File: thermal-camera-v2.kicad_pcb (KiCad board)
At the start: 4 copper layers, 46.3 x 84.7 mm, 121 parts, among them J1 Raspberry_Pi_2_3, J2 Screw_Terminal_M2_L10, J3 Screw_Terminal_M2_L10, J4 Conn_02x04_Odd_Even, J5 Conn_01x03, J6 Screw_Terminal_01x01, U1 ATtiny1616-M, U10 ME6216A28XG, U12 3N25000G33YC, U13 TD6810, U14 TD6810, U15 MMC5633NJL, U16 Ai-Thinker-Ra-01, U2 SHT30-DIS, U3 SIM7600G-H-M.2, U4 ME6211, U5 Flir_LEPTON, U6 SPH0645LM4H, U7 PCF8563T, U8 Antenna_1002427, U9 MAX98357, Y1 Crystal

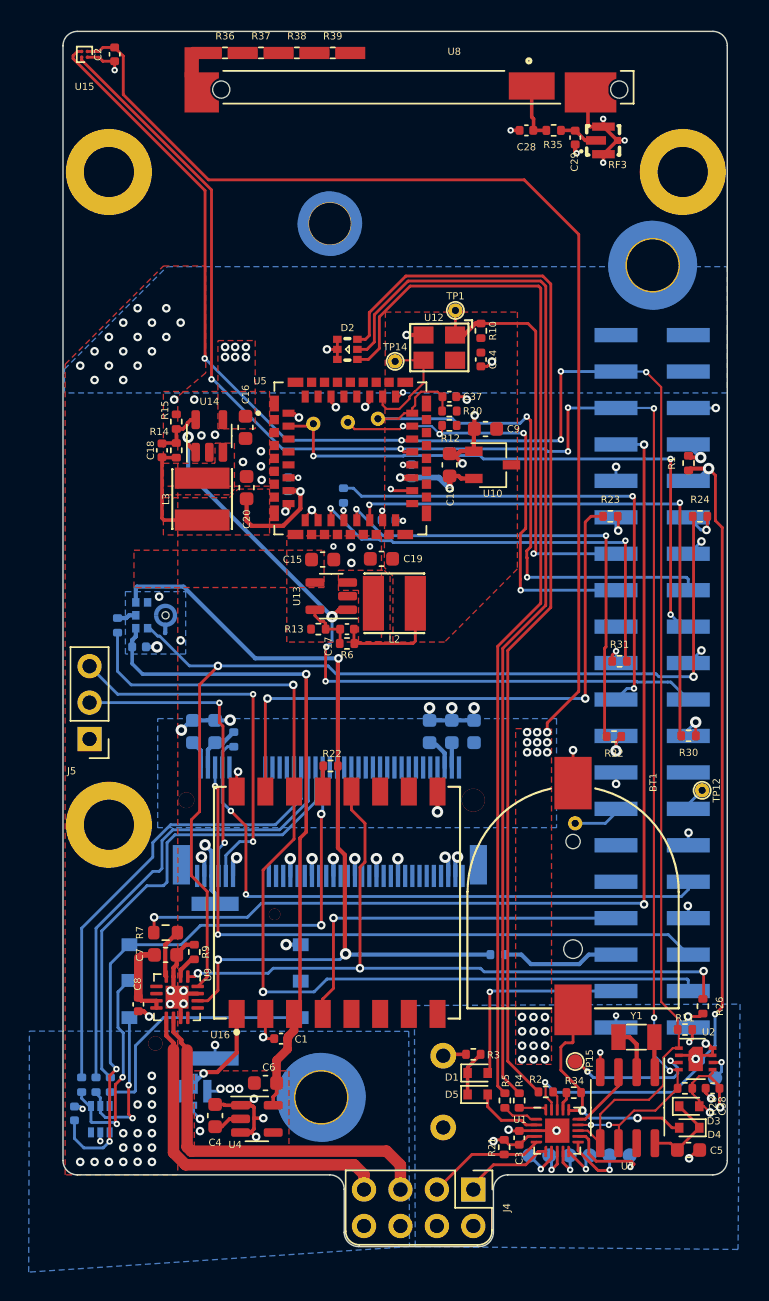
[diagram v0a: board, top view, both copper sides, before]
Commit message: WIP
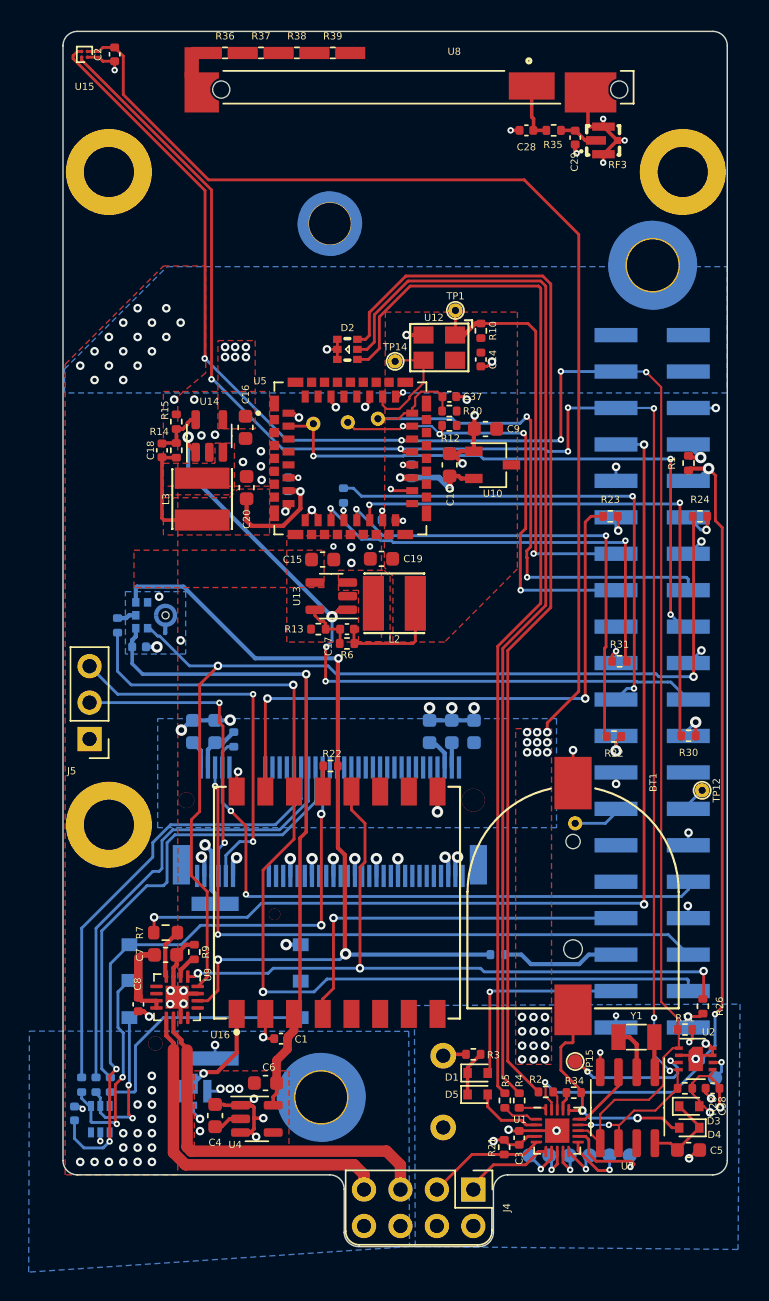
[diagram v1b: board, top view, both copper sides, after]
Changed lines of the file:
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@@
     (pad "32" smd rect (at -3.15 -4.31) (size 0.5 0.84) (layers "F.Cu" "F.Paste" "F.Mask")
       (net 133 "unconnected-(U5-Pad32)") (pinfunction "MIPI_DATA_P") (pintype "output+no_connect"))
+    (model "/home/cam/Downloads/105028-1001.stp"
+      (offset (xyz 0 0 2.1))
+      (scale (xyz 1 1 1))
+      (rotate (xyz -90 0 0))
+    )
   )
   (footprint "cacophony-library:TP" (layer "F.Cu")
@@
       (options (clearance outline) (anchor circle))
       (primitives
-    (gr_arc (start 1.238687 2.158493) (mid 0.331674 1.24433) (end 0 0) (width 1.2))
+    (gr_arc (start 1.238687 2.158493) (mid 0.332763 1.246221) (end 0.000008 0.004362) (width 1.2))
       ))
     (pad "1" smd custom (at 0 -2.5 180) (size 0.1 0.1) (layers "B.Cu" "B.Paste" "B.Mask")
@@
       (options (clearance outline) (anchor circle))
       (primitives
-    (gr_arc (start 1.234921 2.156287) (mid 0.330589 1.242437) (end 0 0) (width 1.2))
+    (gr_arc (start 1.234921 2.156287) (mid 0.332763 1.246219) (end 0.00002 0.008724) (width 1.2))
       ))
     (pad "1" smd custom (at 0 2.5) (size 0.1 0.1) (layers "B.Cu" "B.Paste" "B.Mask")
@@
       (options (clearance outline) (anchor circle))
       (primitives
-    (gr_arc (start 1.238686 2.158492) (mid 0.331673 1.24433) (end 0 0) (width 1.2))
+    (gr_arc (start 1.238686 2.158492) (mid 0.332761 1.246224) (end 0.000004 0.004369) (width 1.2))
       ))
     (pad "1" smd circle (at 0 0 270) (size 6.2 6.2) (layers "B.Cu" "B.Mask")
@@
       (options (clearance outline) (anchor circle))
       (primitives
-    (gr_arc (start 1.234922 2.156288) (mid 0.330589 1.242438) (end 0 0) (width 1.2))
+    (gr_arc (start 1.234922 2.156288) (mid 0.33059 1.242441) (end 0 0.000007) (width 1.2))
       ))
     (pad "1" thru_hole circle (at 0 0 270) (size 3.8 3.8) (drill 3.6) (layers *.Cu *.Mask)
@@
       (rotate (xyz 0 0 0))
     )
-    (model "${CAC_KICAD_LIBRARY}/cacophony-library.3dshapes/RaspberryPi3B.step"
+    (model "${CAC_KICAD_LIBRARY}/cacophony-library.3dshapes/RaspberryPi3B.step" hide
       (offset (xyz 0 0 26))
       (scale (xyz 1 1 1))
@@
       (options (clearance outline) (anchor circle))
       (primitives
-    (gr_arc (start 1.238686 2.158492) (mid 0.331673 1.24433) (end 0 0) (width 1.2))
+    (gr_arc (start 1.238686 2.158492) (mid 0.332761 1.246224) (end 0.000004 0.004369) (width 1.2))
       ))
     (pad "1" smd custom (at -2.5 0 270) (size 0.1 0.1) (layers "B.Cu" "B.Paste" "B.Mask")
@@
       (options (clearance outline) (anchor circle))
       (primitives
-    (gr_arc (start 1.238687 2.158493) (mid 0.331674 1.24433) (end 0 0) (width 1.2))
+    (gr_arc (start 1.238687 2.158493) (mid 0.332763 1.246221) (end 0.000008 0.004362) (width 1.2))
       ))
     (pad "1" smd custom (at 0 -2.5 180) (size 0.1 0.1) (layers "B.Cu" "B.Paste" "B.Mask")
@@
       (options (clearance outline) (anchor circle))
       (primitives
-    (gr_arc (start 1.234921 2.156287) (mid 0.330589 1.242437) (end 0 0) (width 1.2))
+    (gr_arc (start 1.234921 2.156287) (mid 0.332763 1.246219) (end 0.00002 0.008724) (width 1.2))
       ))
     (pad "1" thru_hole circle (at 0 0 270) (size 3.8 3.8) (drill 3.6) (layers *.Cu *.Mask)
@@
       (options (clearance outline) (anchor circle))
       (primitives
-    (gr_arc (start 1.234922 2.156288) (mid 0.330589 1.242438) (end 0 0) (width 1.2))
+    (gr_arc (start 1.234922 2.156288) (mid 0.33059 1.242441) (end 0 0.000007) (width 1.2))
       ))
     (model "${CAC_KICAD_LIBRARY}/cacophony-library.3dshapes/SMD_BD4.4-L4.4-D2.8.wrl"
@@
   (gr_arc (start 130.8 135.4) (mid 130.507107 136.107107) (end 129.8 136.4) (layer "Edge.Cuts") (width 0.1))
   (gr_arc (start 147.1 130.4) (mid 146.807107 131.107107) (end 146.1 131.4) (layer "Edge.Cuts") (width 0.1))
+  (dimension (type aligned) (layer "User.2")
+    (pts (xy 144 61.5) (xy 104 61.5))
+    (height 22.95)
+    (gr_text "40.0000 mm" (at 124 37.4) (layer "User.2")
+      (effects (font (size 1 1) (thickness 0.15)))
+    )
+    (format (units 3) (units_format 1) (precision 4))
+    (style (thickness 0.15) (arrow_length 1.27) (text_position_mode 0) (extension_height 0.58642) (extension_offset 0.5) keep_text_aligned)
+  )
+  (dimension (type aligned) (layer "User.2")
+    (pts (xy 104 61.5) (xy 104 107))
+    (height 21.299999)
+    (gr_text "45.5000 mm" (at 81.550001 84.25 90) (layer "User.2")
+      (effects (font (size 1 1) (thickness 0.15)))
+    )
+    (format (units 3) (units_format 1) (precision 4))
+    (style (thickness 0.15) (arrow_length 1.27) (text_position_mode 0) (extension_height 0.58642) (extension_offset 0.5) keep_text_aligned)
+  )
   (dimension (type orthogonal) (layer "User.2")
     (pts (xy 100.8 52.7) (xy 147.1 52.7))
